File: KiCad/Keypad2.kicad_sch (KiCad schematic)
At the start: 17 parts, among them J1 Keypad, J2 Prog, U1 SP3485, U2 ESP32-PICO-MINI-02, U3 LMR16006+FB

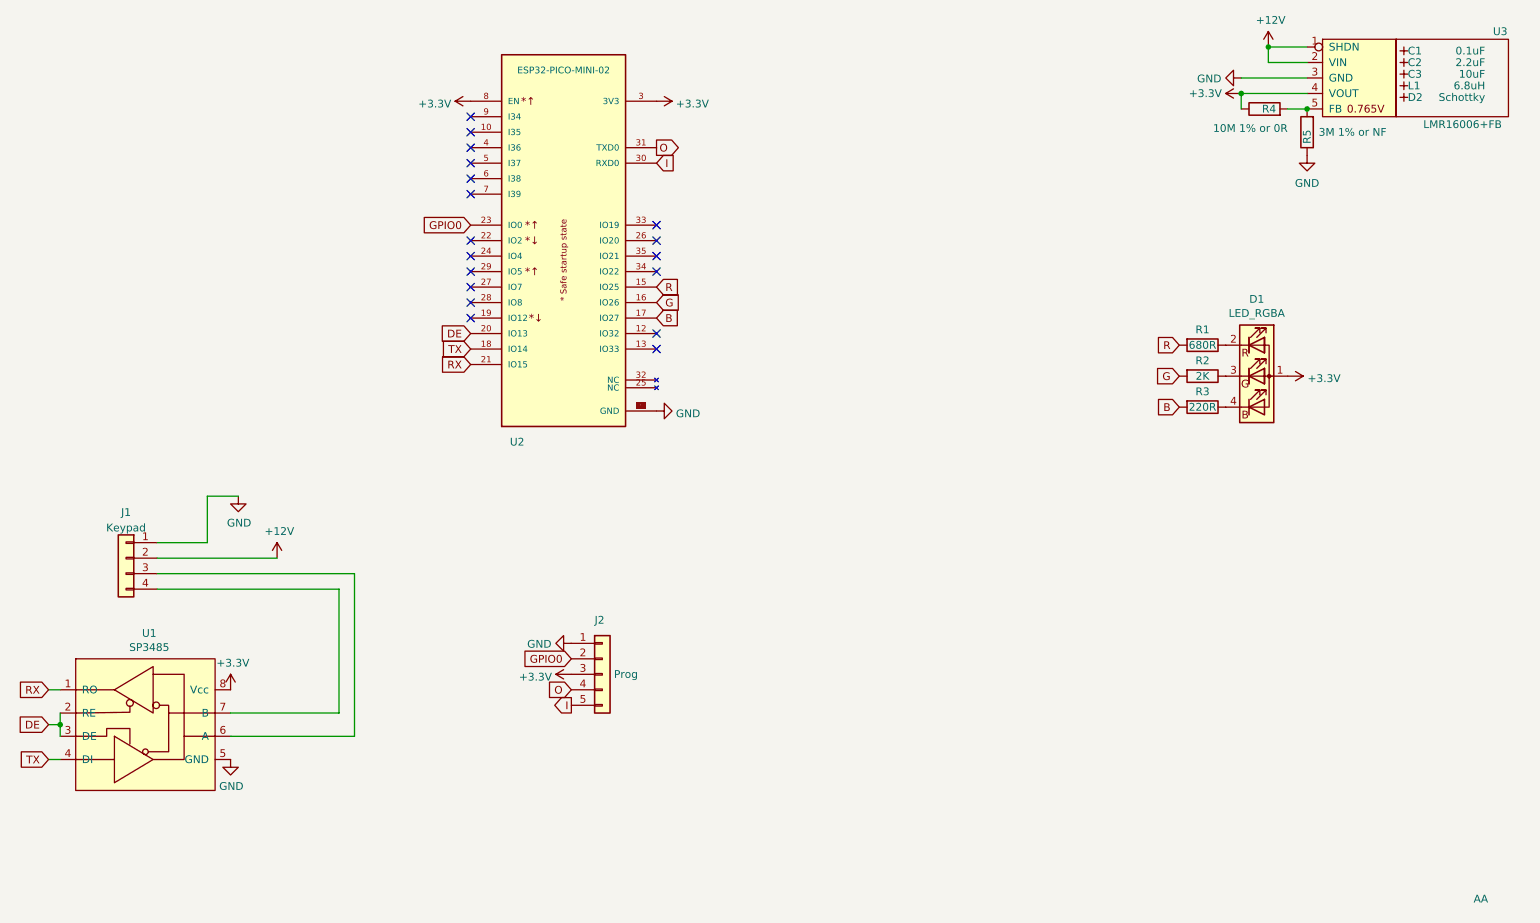
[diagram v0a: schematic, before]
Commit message: Clean up
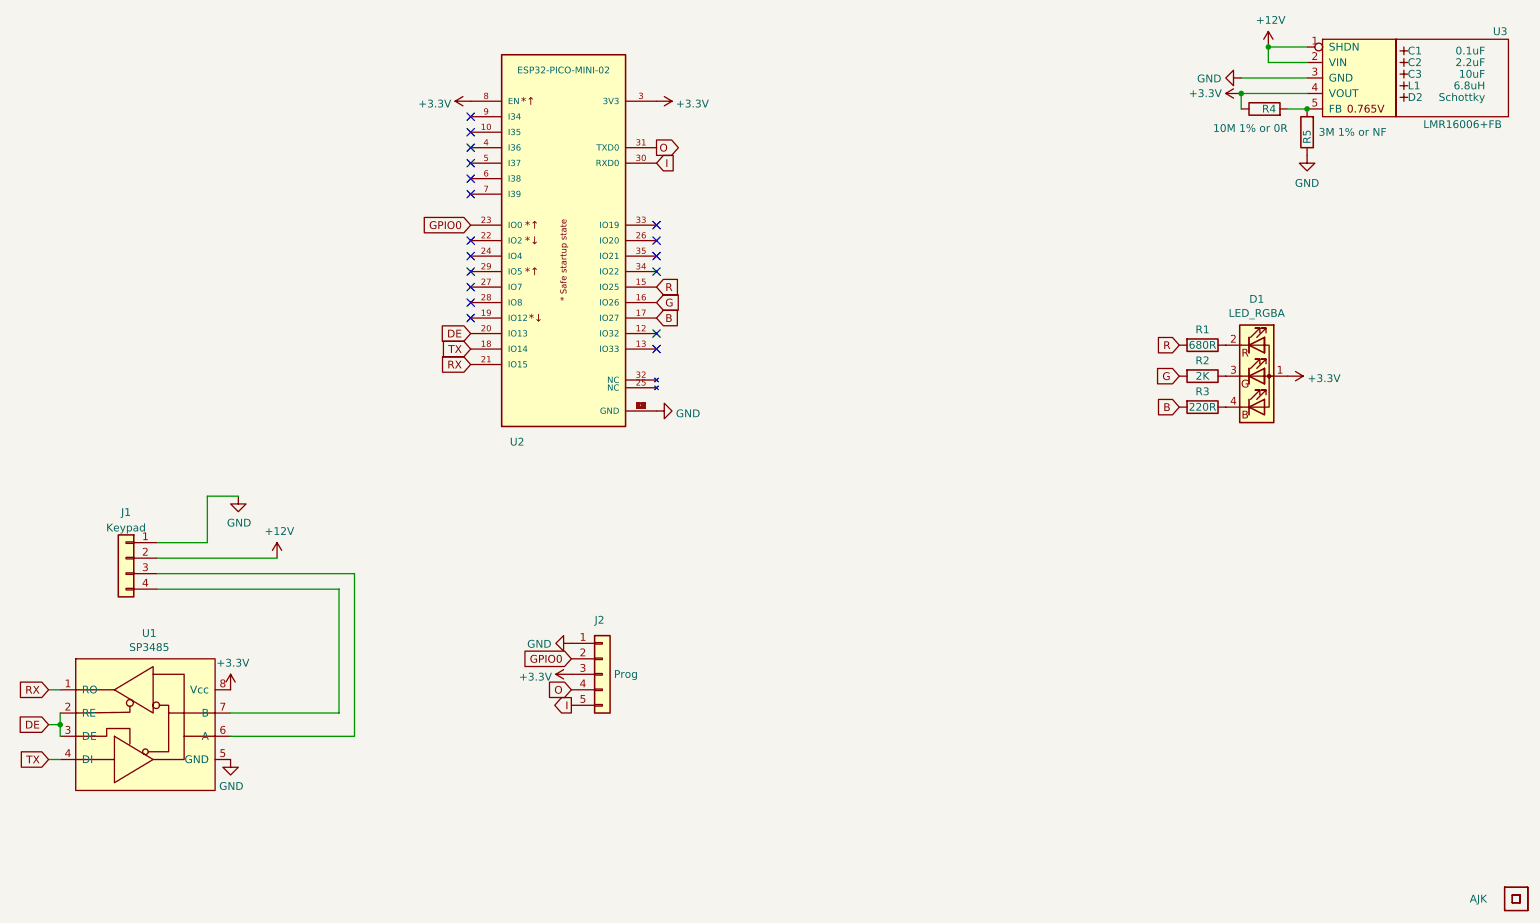
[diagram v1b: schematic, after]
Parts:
- removed Logo1: AA, RevK:AA, symbol RevK:AA
- added Logo1: AJK, RevK:AJK, symbol RevK:AJK
- added U4: QR, RevK:QR-SS, symbol RevK:QR
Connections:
- net GND: no longer U2.54 (GND), U2.55 (GND), U2.56 (GND), U2.57 (GND), U2.58 (GND), U2.59 (GND), U2.60 (GND), U2.61 (GND)
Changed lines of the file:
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@@
     (pin "1")
-  )
-  (symbol (lib_id "RevK:AA") (at 266.7 172.72 0) (unit 1)
-    (in_bom yes) (on_board yes)
-    (property "Reference" "Logo1" (id 0) (at 266.7 172.72 0)
-      (effects (font (size 1.27 1.27)) hide)
-    )
-    (property "Value" "AA" (id 1) (at 267.335 172.72 0)
-      (effects (font (size 1.27 1.27)) (justify left))
-    )
-    (property "Footprint" "RevK:AA" (id 2) (at 266.7 172.72 0)
-      (effects (font (size 1.27 1.27)) hide)
-    )
-    (property "Datasheet" "" (id 3) (at 266.7 172.72 0)
-      (effects (font (size 1.27 1.27)) hide)
-    )
-    (property "Note" "Non part, PCB printed" (id 4) (at 266.7 172.72 0)
-      (effects (font (size 1.27 1.27)) hide)
-    )
   )
   (symbol (lib_id "power:+12V") (at 71.12 116.84 0) (unit 1)
@@
     (pin "1")
   )
+  (symbol (lib_id "RevK:QR") (at 274.32 172.72 0) (unit 1)
+    (in_bom no) (on_board yes) (fields_autoplaced)
+    (property "Reference" "U4" (id 0) (at 274.32 175.895 0)
+      (effects (font (size 1.27 1.27)) hide)
+    )
+    (property "Value" "QR" (id 1) (at 274.32 175.895 0)
+      (effects (font (size 1.27 1.27)) hide)
+    )
+    (property "Footprint" "RevK:QR-SS" (id 2) (at 273.685 173.355 0)
+      (effects (font (size 1.27 1.27)) hide)
+    )
+    (property "Datasheet" "" (id 3) (at 273.685 173.355 0)
+      (effects (font (size 1.27 1.27)) hide)
+    )
+    (property "Note" "Non part, PCB printed" (id 4) (at 274.32 172.72 0)
+      (effects (font (size 1.27 1.27)) hide)
+    )
+  )
   (symbol (lib_id "power:GND") (at 240.03 50.8 0) (unit 1)
     (in_bom yes) (on_board yes) (fields_autoplaced)
@@
       (effects (font (size 1.27 1.27)) (justify left))
     )
-    (property "Footprint" "Connector_PinHeader_2.54mm:PinHeader_1x05_P2.54mm_Vertical" (id 2) (at 124.46 135.89 0)
+    (property "Footprint" "Connector_PinHeader_2.54mm:PinHeader_1x05_P2.54mm_Vertical" (id 2) (at 124.46 143.51 0)
       (effects (font (size 1.27 1.27)) hide)
     )
@@
     (pin "52")
     (pin "53")
-    (pin "54")
-    (pin "55")
-    (pin "56")
-    (pin "57")
-    (pin "58")
-    (pin "59")
     (pin "6")
-    (pin "60")
-    (pin "61")
     (pin "7")
     (pin "8")
@@
     )
     (pin "1")
+  )
+  (symbol (lib_id "RevK:AJK") (at 269.24 172.72 0) (unit 1)
+    (in_bom no) (on_board yes)
+    (property "Reference" "Logo1" (id 0) (at 269.24 170.18 0)
+      (effects (font (size 1.27 1.27)) hide)
+    )
+    (property "Value" "AJK" (id 1) (at 266.7 172.72 0)
+      (effects (font (size 1.27 1.27)) (justify left))
+    )
+    (property "Footprint" "RevK:AJK" (id 2) (at 269.24 175.26 0)
+      (effects (font (size 1.27 1.27)) hide)
+    )
+    (property "Datasheet" "" (id 3) (at 269.24 175.26 0)
+      (effects (font (size 1.27 1.27)) hide)
+    )
+    (property "Note" "Non part, PCB printed" (id 4) (at 269.24 172.72 0)
+      (effects (font (size 1.27 1.27)) hide)
+    )
   )
   (symbol (lib_id "power:+12V") (at 233.68 33.02 0) (unit 1)
@@
     (property "Reference" "J1" (id 0) (at 46.355 109.3302 0))
     (property "Value" "Keypad" (id 1) (at 46.355 111.8671 0))
-    (property "Footprint" "RevK:Molex_MiniSPOX_H4V" (id 2) (at 46.355 116.84 0)
+    (property "Footprint" "RevK:Molex_MiniSPOX_H4V" (id 2) (at 46.355 124.46 0)
       (effects (font (size 1.27 1.27)) hide)
     )
@@
       (reference "L1") (unit 1) (value "6.8uH") (footprint "RevK:Hidden")
     )
-    (path "/00000000-0000-0000-0000-000060b9351c"
-      (reference "Logo1") (unit 1) (value "AA") (footprint "RevK:AA")
+    (path "/d8b4cc04-1cc7-43a2-af9d-685210cb4548"
+      (reference "Logo1") (unit 1) (value "AJK") (footprint "RevK:AJK")
     )
     (path "/00000000-0000-0000-0000-000060ce4fe8"
@@
       (reference "U3") (unit 1) (value "LMR16006+FB") (footprint "RevK:RegulatorBlockFB")
     )
-  )
+    (path "/31b42c3f-ef68-4fb7-bba0-44bb7a0027da"
+      (reference "U4") (unit 1) (value "QR") (footprint "RevK:QR-SS")
+    )
+  )
